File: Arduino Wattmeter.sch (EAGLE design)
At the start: 25 parts, among them U1 328P, U2 AP2202-ADJ, U3 LF398, U4 LF398

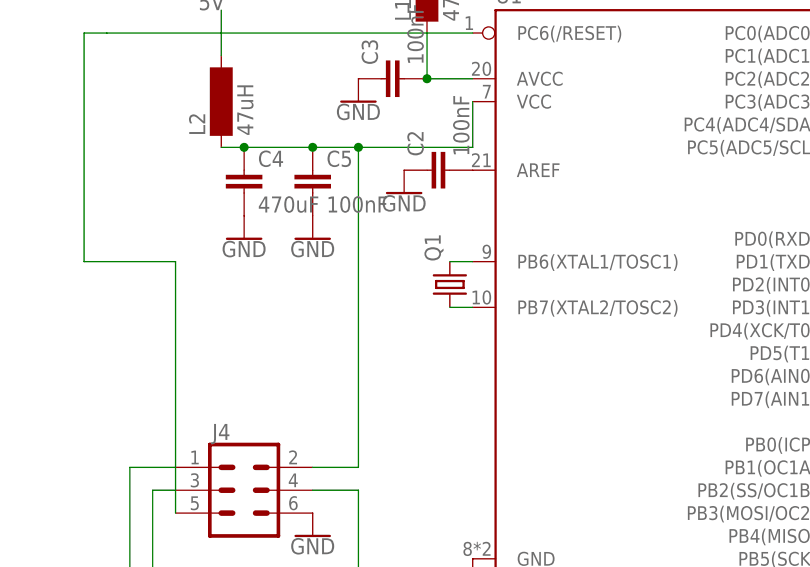
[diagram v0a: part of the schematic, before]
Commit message: fixed with via
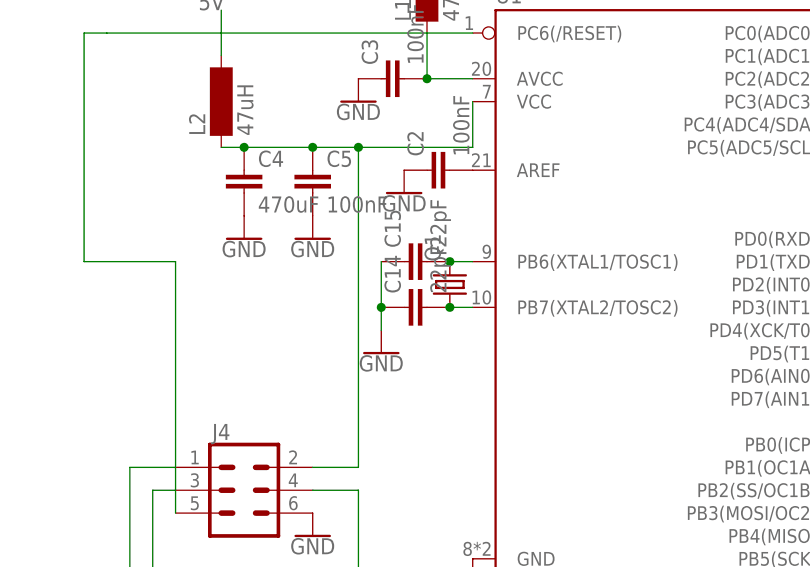
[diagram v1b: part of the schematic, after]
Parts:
- added C14, C15: 22pF, SparkFun-Capacitors:1.0UF-1206-50V-10%
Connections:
- net GND: now also C14.1, C15.1
- net N$2: now also C15.2
- net N$3: now also C14.2
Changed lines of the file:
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@@
 <part name="J3" library="SparkFun-Connectors" deviceset="CONN_04" device=""/>
 <part name="J5" library="SparkFun-Connectors" deviceset="CONN_04" device=""/>
+<part name="C14" library="SparkFun-Capacitors" deviceset="1.0UF" device="-1206-50V-10%" value="22pF"/>
+<part name="C15" library="SparkFun-Capacitors" deviceset="1.0UF" device="-1206-50V-10%" value="22pF"/>
+<part name="GND12" library="SparkFun-PowerSymbols" deviceset="GND" device=""/>
 </parts>
 <sheets>
@@
 <instance part="J3" gate="G$1" x="172.72" y="121.92" rot="R180"/>
 <instance part="J5" gate="G$1" x="-93.98" y="121.92"/>
+<instance part="C14" gate="G$1" x="-17.78" y="101.6" rot="R90"/>
+<instance part="C15" gate="G$1" x="-17.78" y="106.68" rot="R90"/>
+<instance part="GND12" gate="1" x="-22.86" y="96.52"/>
 </instances>
 <busses>
@@
 <wire x1="-88.9" y1="124.46" x2="-81.28" y2="124.46" width="0.1524" layer="91"/>
 <label x="-78.74" y="124.46" size="1.778" layer="95"/>
+</segment>
+<segment>
+<pinref part="C15" gate="G$1" pin="1"/>
+<wire x1="-22.86" y1="106.68" x2="-22.86" y2="101.6" width="0.1524" layer="91"/>
+<pinref part="C14" gate="G$1" pin="1"/>
+<wire x1="-22.86" y1="101.6" x2="-22.86" y2="99.06" width="0.1524" layer="91"/>
+<junction x="-22.86" y="101.6"/>
+<pinref part="GND12" gate="1" pin="GND"/>
 </segment>
 </net>
@@
 <pinref part="Q1" gate="G$1" pin="2"/>
 <wire x1="-12.7" y1="106.68" x2="-15.24" y2="106.68" width="0.1524" layer="91"/>
+<pinref part="C15" gate="G$1" pin="2"/>
+<junction x="-15.24" y="106.68"/>
 </segment>
 </net>
@@
 <pinref part="Q1" gate="G$1" pin="1"/>
 <wire x1="-12.7" y1="101.6" x2="-15.24" y2="101.6" width="0.1524" layer="91"/>
-</segment>
-</net>
+<pinref part="C14" gate="G$1" pin="2"/>
+<junction x="-15.24" y="101.6"/>
+</segment>
+</net>
